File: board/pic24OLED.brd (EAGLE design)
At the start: 100 x 80 mm, 10 parts, among them U1 PIC24FJ64GA002T-I/ML

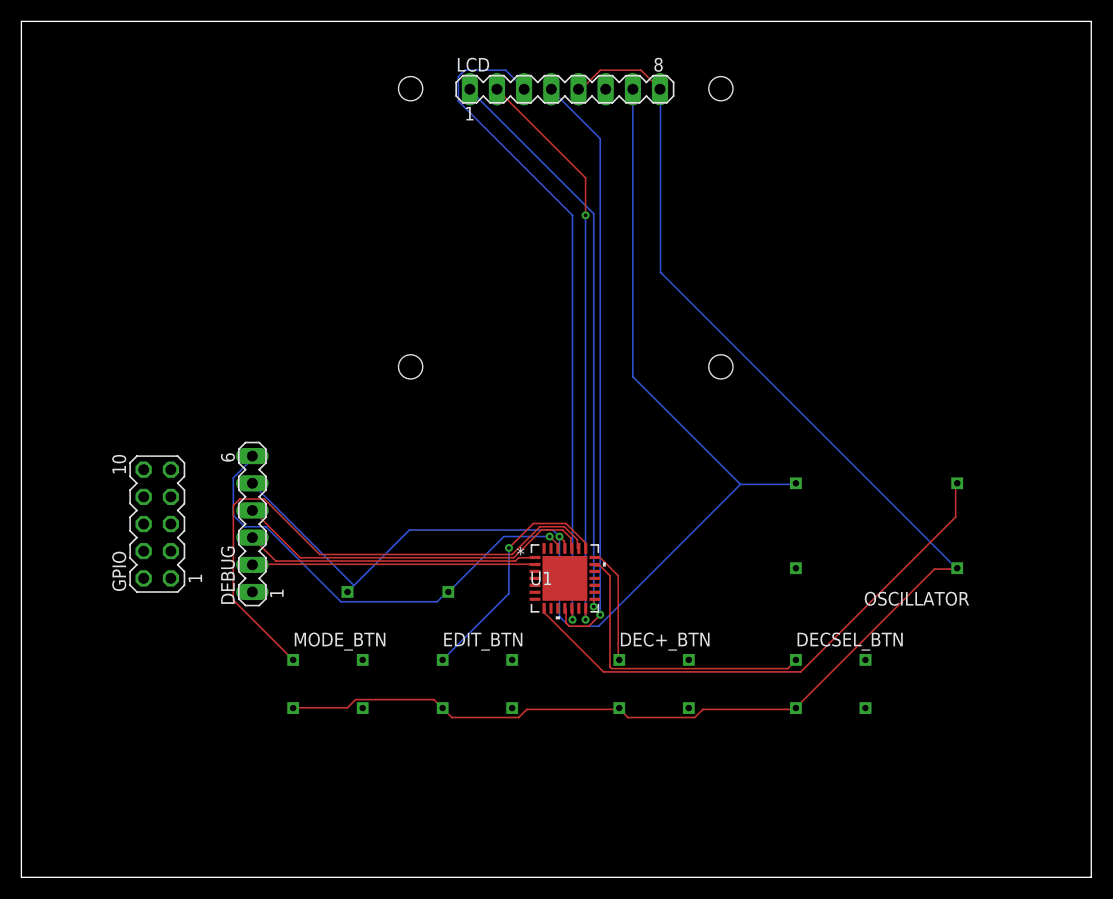
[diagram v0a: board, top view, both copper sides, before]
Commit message: Finished up first board draft completely.
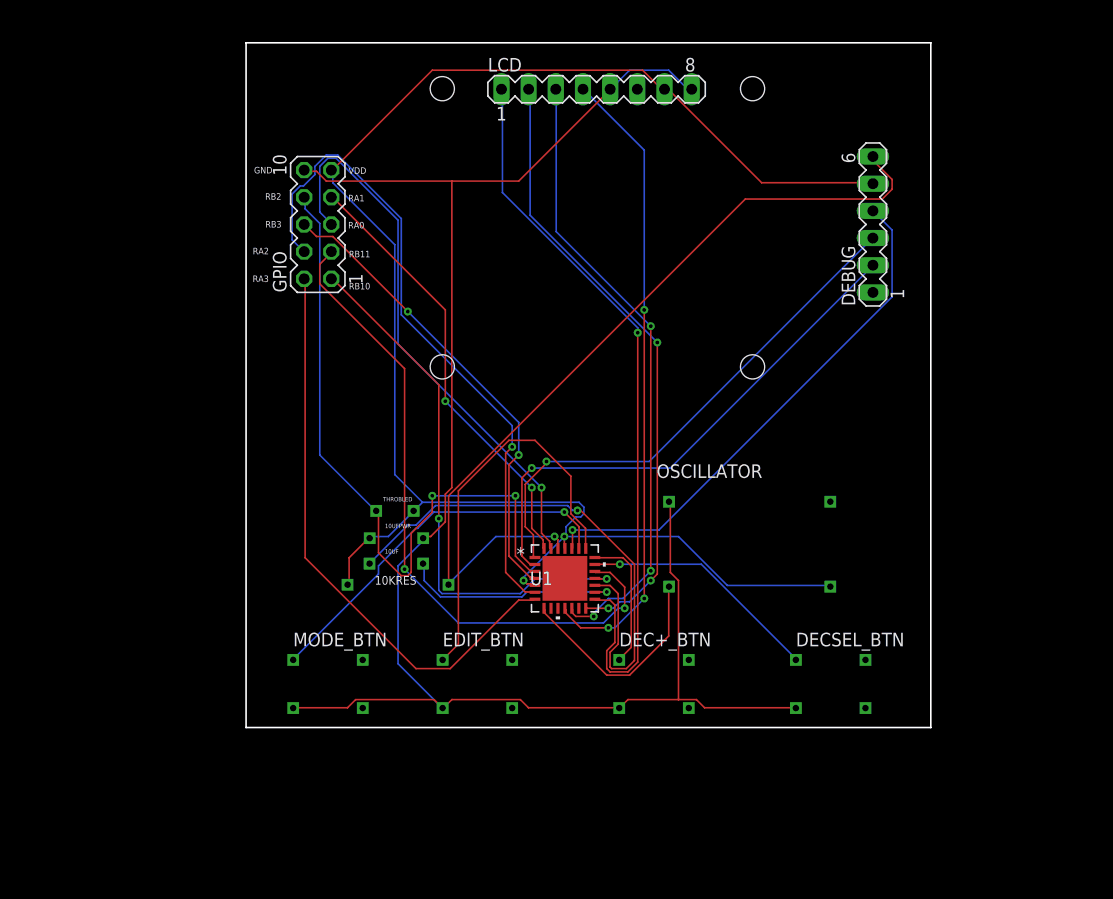
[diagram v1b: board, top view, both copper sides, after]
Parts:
- removed U$1: THRESISTOR, pic24fj64ga002:THRESISTOR
- added 10KRES: THRESISTOR, pic24fj64ga002:THRESISTOR
- added 10UF, 10UFPWR: THCAP, pic24fj64ga002:THCAP
- added THROBLED: THLED, pic24fj64ga002:THLED
- moved DEBUG 64.4 mm to (79.6, 61.0)
- moved GPIO 31.8 mm to (27.7, 61.0)
- moved OSCILLATOR 10.2 mm to (75.6, 27.2), turned to 180 degrees
- moved LCD 2.96 mm to (53.8, 73.7)
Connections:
- new net N$22: 10UF.P$1, U1.17
- new net N$23: 10UF.P$2, U1.16
- net GND: now also 10UFPWR.P$2
- net N$13: now also 10KRES.P$2; no longer U$1.P$2
- net N$14: now also THROBLED.GND
- net VDD: now also 10KRES.P$1, 10UFPWR.P$1, THROBLED.PWR, U1.5; no longer U$1.P$1
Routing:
- net N$14: track 0.00 -> 64.0 mm, vias 0 -> 2
- net N$20: track 0.00 -> 62.0 mm, vias 0 -> 2
- net N$16: track 0.00 -> 61.6 mm, vias 0 -> 1
- net N$17: track 0.00 -> 54.6 mm
- net N$19: track 0.00 -> 52.5 mm, vias 0 -> 1
- net N$21: track 0.00 -> 50.9 mm, vias 0 -> 2
- net N$22: track 0.00 -> 50.6 mm, vias 0 -> 1
- net VDD: track 113.9 -> 159.1 mm, vias 1 -> 3
- net N$15: track 0.00 -> 43.9 mm, vias 0 -> 2
- net N$18: track 0.00 -> 41.1 mm, vias 0 -> 2
- net N$13: track 43.2 -> 78.6 mm, vias 1 -> 2
- net N$7: track 50.4 -> 20.6 mm
- net GND: track 135.1 -> 163.0 mm
- net N$2: track 26.4 -> 49.9 mm, vias 0 -> 2
- net N$6: track 27.4 -> 49.3 mm, vias 0 -> 2
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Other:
- board size 100 x 80 mm -> 64 x 64 mm
- board text added: "GND"
- board text added: "Loubear - June 2019 louisbarrett98@gmail.com"
- board text added: "RA0"
- board text added: "RA1"
- board text added: "RA2"
- board text added: "RA3"
- board text added: "RB10"
- board text added: "RB11"
- board text added: "RB2"
- board text added: "RB3"
- board text added: "VDD"
